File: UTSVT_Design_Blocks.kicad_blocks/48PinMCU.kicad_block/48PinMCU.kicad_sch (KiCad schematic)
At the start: 29 parts, among them J1 SWD_Header_02x02, SW1 SW_SPDT, SW2 Reset, U1 STM32G431CBT6, Y1 Crystal

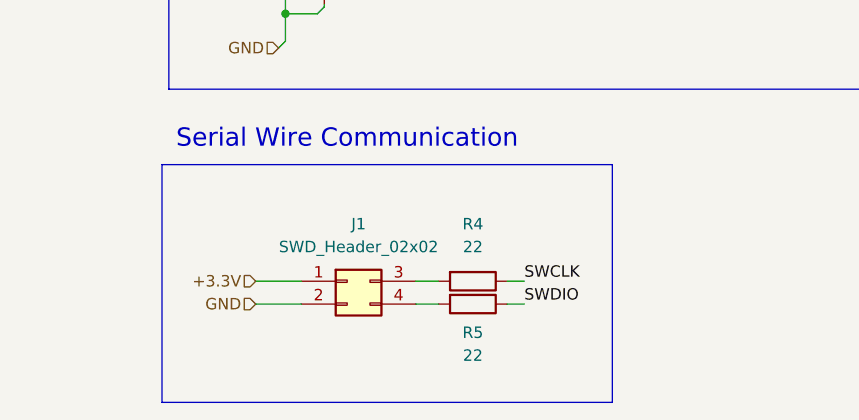
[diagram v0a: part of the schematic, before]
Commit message: jk I'm still a chud
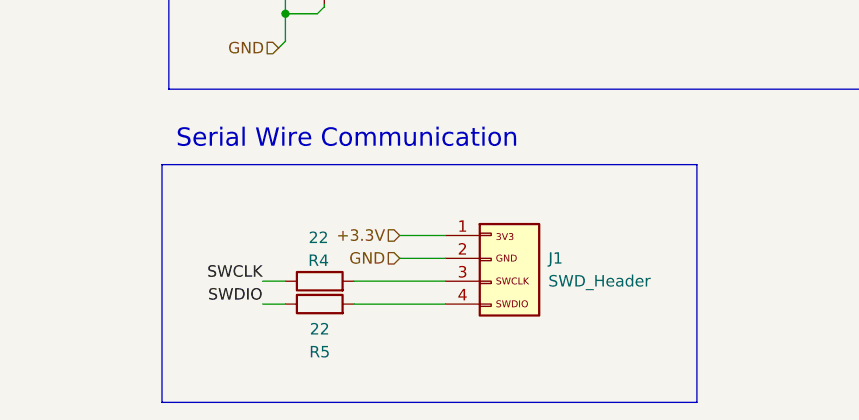
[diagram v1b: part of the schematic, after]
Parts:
- removed J1: SWD_Header_02x02, 878320406:CONN04_878320406_MOL, symbol 100PinMCU:SWD_Header_02x02
- added J1: SWD_Header, UTSVT_Connectors:SWD_Conn, symbol utsvt_connectors:SWD_Header
- SW1: footprint BootSW:BootSW -> UTSVT_Special:BootSW
- Y1: footprint Crystal:Crystal_SMD_Abracon_ABM3-2Pin_5.0x3.2mm -> UTSVT_Passives:Crystal_SMD_Abracon_ABM3-2Pin_5.0x3.2mm
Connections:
- net +3.3V: now also J1.1 (Pin_1)
- net GND: now also J1.2 (Pin_2)
- net at R4.2: now also J1.3 (Pin_3)
- net at R5.2: now also J1.4 (Pin_4)
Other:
- moved on the sheet: R4, R5
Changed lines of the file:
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@@
 	(rectangle
 		(start 164.084 134.366)
-		(end 214.122 160.782)
+		(end 223.52 160.782)
 		(stroke
 			(width 0)
@@
 	(wire
 		(pts
-			(xy 202.438 149.86) (xy 204.343 149.86)
+			(xy 177.8 149.86) (xy 175.26 149.86)
 		)
 		(stroke
@@
 	(wire
 		(pts
-			(xy 174.498 149.86) (xy 179.578 149.86)
+			(xy 190.5 144.78) (xy 195.58 144.78)
 		)
 		(stroke
@@
 	(wire
 		(pts
-			(xy 192.278 149.86) (xy 194.818 149.86)
+			(xy 185.42 149.86) (xy 195.58 149.86)
 		)
 		(stroke
@@
 	(wire
 		(pts
-			(xy 202.438 147.32) (xy 204.343 147.32)
+			(xy 177.8 147.32) (xy 175.26 147.32)
 		)
 		(stroke
@@
 	(wire
 		(pts
-			(xy 192.278 147.32) (xy 194.818 147.32)
+			(xy 195.58 147.32) (xy 185.42 147.32)
 		)
 		(stroke
@@
 	(wire
 		(pts
-			(xy 174.498 147.32) (xy 179.578 147.32)
+			(xy 190.5 142.24) (xy 195.58 142.24)
 		)
 		(stroke
@@
 	)
 	(label "SWCLK"
-		(at 204.343 147.32 0)
+		(at 175.26 147.32 180)
 		(effects
 			(font
 				(size 1.27 1.27)
 			)
-			(justify left bottom)
+			(justify right bottom)
 		)
 	)
@@
 	)
 	(label "SWDIO"
-		(at 204.343 149.86 0)
+		(at 175.26 149.86 180)
 		(effects
 			(font
 				(size 1.27 1.27)
 			)
-			(justify left bottom)
+			(justify right bottom)
 		)
 	)
@@
 	(hierarchical_label "GND"
 		(shape input)
-		(at 174.498 149.86 180)
+		(at 190.5 144.78 180)
 		(effects
 			(font
@@
 	(hierarchical_label "+3.3V"
 		(shape input)
-		(at 174.498 147.32 180)
+		(at 190.5 142.24 180)
 		(effects
 			(font
@@
 			)
 		)
-		(property "Footprint" "Crystal:Crystal_SMD_Abracon_ABM3-2Pin_5.0x3.2mm"
+		(property "Footprint" "UTSVT_Passives:Crystal_SMD_Abracon_ABM3-2Pin_5.0x3.2mm"
 			(at 134.62 91.948 0)
 			(effects
@@
 	(symbol
 		(lib_id "Device:R")
-		(at 198.628 147.32 270)
+		(at 181.61 147.32 90)
 		(unit 1)
 		(exclude_from_sim no)
@@
 		(on_board yes)
 		(dnp no)
-		(fields_autoplaced yes)
 		(property "Reference" "R4"
-			(at 198.628 140.97 90)
+			(at 181.483 145.034 90)
 			(effects
 				(font
@@
 		)
 		(property "Value" "22"
-			(at 198.628 143.51 90)
+			(at 181.483 142.494 90)
 			(effects
 				(font
@@
 		)
 		(property "Footprint" "Resistor_SMD:R_0603_1608Metric_Pad0.98x0.95mm_HandSolder"
-			(at 198.628 145.542 90)
+			(at 181.61 149.098 90)
 			(effects
 				(font
@@
 		)
 		(property "Datasheet" "~"
-			(at 198.628 147.32 0)
+			(at 181.61 147.32 0)
 			(effects
 				(font
@@
 		)
 		(property "Description" "Resistor"
-			(at 198.628 147.32 0)
+			(at 181.61 147.32 0)
 			(effects
 				(font
@@
 		)
 		(property "LCSC P/N" "C2930077"
-			(at 198.628 147.32 90)
+			(at 181.61 147.32 90)
 			(effects
 				(font
@@
 		)
 		(property "LSCS P/N" ""
-			(at 198.628 147.32 90)
+			(at 181.61 147.32 90)
 			(effects
 				(font
@@
 		)
 		(property "P/N" "FRC0603F22R0TS"
-			(at 198.628 147.32 90)
+			(at 181.61 147.32 90)
 			(effects
 				(font
@@
 	(symbol
 		(lib_id "Device:R")
-		(at 198.628 149.86 270)
+		(at 181.61 149.86 90)
 		(unit 1)
 		(exclude_from_sim no)
@@
 		(dnp no)
 		(property "Reference" "R5"
-			(at 198.628 153.035 90)
+			(at 181.61 155.194 90)
 			(effects
 				(font
@@
 		)
 		(property "Value" "22"
-			(at 198.628 155.575 90)
+			(at 181.61 152.654 90)
 			(effects
 				(font
@@
 		)
 		(property "Footprint" "Resistor_SMD:R_0603_1608Metric_Pad0.98x0.95mm_HandSolder"
-			(at 198.628 148.082 90)
+			(at 181.61 151.638 90)
 			(effects
 				(font
@@
 		)
 		(property "Datasheet" "~"
-			(at 198.628 149.86 0)
+			(at 181.61 149.86 0)
 			(effects
 				(font
@@
 		)
 		(property "Description" "Resistor"
-			(at 198.628 149.86 0)
+			(at 181.61 149.86 0)
 			(effects
 				(font
@@
 		)
 		(property "LCSC P/N" "C2930077"
-			(at 198.628 149.86 90)
+			(at 181.61 149.86 90)
 			(effects
 				(font
@@
 		)
 		(property "LSCS P/N" ""
-			(at 198.628 149.86 90)
+			(at 181.61 149.86 90)
 			(effects
 				(font
@@
 		)
 		(property "P/N" "FRC0603F22R0TS"
-			(at 198.628 149.86 90)
+			(at 181.61 149.86 90)
 			(effects
 				(font
@@
 			)
 		)
-		(property "Footprint" "BootSW:BootSW"
+		(property "Footprint" "UTSVT_Special:BootSW"
 			(at 231.14 102.362 0)
 			(effects
@@
 	)
 	(symbol
+		(lib_id "utsvt_connectors:SWD_Header")
+		(at 199.39 142.24 0)
+		(unit 1)
+		(exclude_from_sim no)
+		(in_bom yes)
+		(on_board yes)
+		(dnp no)
+		(fields_autoplaced yes)
+		(property "Reference" "J1"
+			(at 207.01 144.7799 0)
+			(effects
+				(font
+					(size 1.27 1.27)
+				)
+				(justify left)
+			)
+		)
+		(property "Value" "SWD_Header"
+			(at 207.01 147.3199 0)
+			(effects
+				(font
+					(size 1.27 1.27)
+				)
+				(justify left)
+			)
+		)
+		(property "Footprint" "UTSVT_Connectors:SWD_Conn"
+			(at 199.39 142.24 0)
+			(effects
+				(font
+					(size 1.27 1.27)
+				)
+				(hide yes)
+			)
+		)
+		(property "Datasheet" "kicad-embed://Conn_02x02_Odd_Even.pdf"
+			(at 199.39 142.24 0)
+			(effects
+				(font
+					(size 1.27 1.27)
+				)
+				(hide yes)
+			)
+		)
+		(property "Description" "Generic connector, double row, 02x02"
+			(at 199.39 142.24 0)
+			(effects
+				(font
+					(size 1.27 1.27)
+				)
+				(hide yes)
+			)
+		)
+		(property "P/N" "0878320406"
+			(at 199.39 142.24 0)
+			(effects
+				(font
+					(size 1.27 1.27)
+				)
+				(hide yes)
+			)
+		)
+		(property "LSCS P/N" "C17492485"
+			(at 199.39 142.24 0)
+			(effects
+				(font
+					(size 1.27 1.27)
+				)
+				(hide yes)
+			)
+		)
+		(pin "1"
+		)
+		(pin "2"
+		)
+		(pin "3"
+		)
+		(pin "4"
+		)
+		(instances
+			(project ""
+				(path "/b973e36d-c926-4cad-b0c3-dce51444ffeb"
+					(reference "J1")
+					(unit 1)
+				)
+			)
+		)
+	)
+	(symbol
 		(lib_id "Device:R")
 		(at 248.92 107.442 180)
@@
 					(unit 1)
 				)
-			)
-		)
-	)
-	(symbol
-		(lib_id "100PinMCU:SWD_Header_02x02")
-		(at 184.658 147.32 0)
-		(unit 1)
-		(exclude_from_sim no)
-		(in_bom yes)
-		(on_board yes)
-		(dnp no)
-		(fields_autoplaced yes)
-		(property "Reference" "J1"
-			(at 185.928 140.97 0)
-			(effects
-				(font
-					(size 1.27 1.27)
-				)
-			)
-		)
-		(property "Value" "SWD_Header_02x02"
-			(at 185.928 143.51 0)
-			(effects
-				(font
-					(size 1.27 1.27)
-				)
-			)
-		)
-		(property "Footprint" "878320406:CONN04_878320406_MOL"
-			(at 184.658 147.32 0)
-			(effects
-				(font
-					(size 1.27 1.27)
-				)
-				(hide yes)
-			)
-		)
-		(property "Datasheet" "kicad-embed://Conn_02x02_Odd_Even.pdf"
-			(at 184.658 147.32 0)
-			(effects
-				(font
-					(size 1.27 1.27)
-				)
-				(hide yes)
-			)
-		)
-		(property "Description" "Generic connector, double row, 02x02, odd/even pin numbering scheme (row 1 odd numbers, row 2 even numbers), script generated (kicad-library-utils/schlib/autogen/connector/)"
-			(at 184.658 147.32 0)
-			(effects
-				(font
-					(size 1.27 1.27)
-				)
-				(hide yes)
-			)
-		)
-		(property "P/N" "0878320406"
-			(at 184.658 147.32 0)
-			(effects
-				(font
-					(size 1.27 1.27)
-				)
-				(hide yes)
-			)
-		)
-		(property "LCSC P/N" "C17492485"
-			(at 184.658 147.32 0)
-			(effects
-				(font
-					(size 1.27 1.27)
-				)
-				(hide yes)
-			)
-		)
-		(property "LSCS P/N" ""
-			(at 184.658 147.32 0)
-			(effects
-				(font
-					(size 1.27 1.27)
-				)
-				(hide yes)
-			)
-		)
-		(pin "2"
-		)
-		(pin "1"
-		)
-		(pin "4"
-		)
-		(pin "3"
-		)
-		(instances
-			(project "48PinMCU"
-				(path "/b973e36d-c926-4cad-b0c3-dce51444ffeb"
-					(reference "J1")
-					(unit 1)
-				)
